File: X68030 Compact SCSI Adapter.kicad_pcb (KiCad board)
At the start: 2 copper layers, 28.8 x 85.3 mm, 5 parts, among them J1 X68030 Internal SCSI Connector, J2 DB25_Plug_MountingHoles

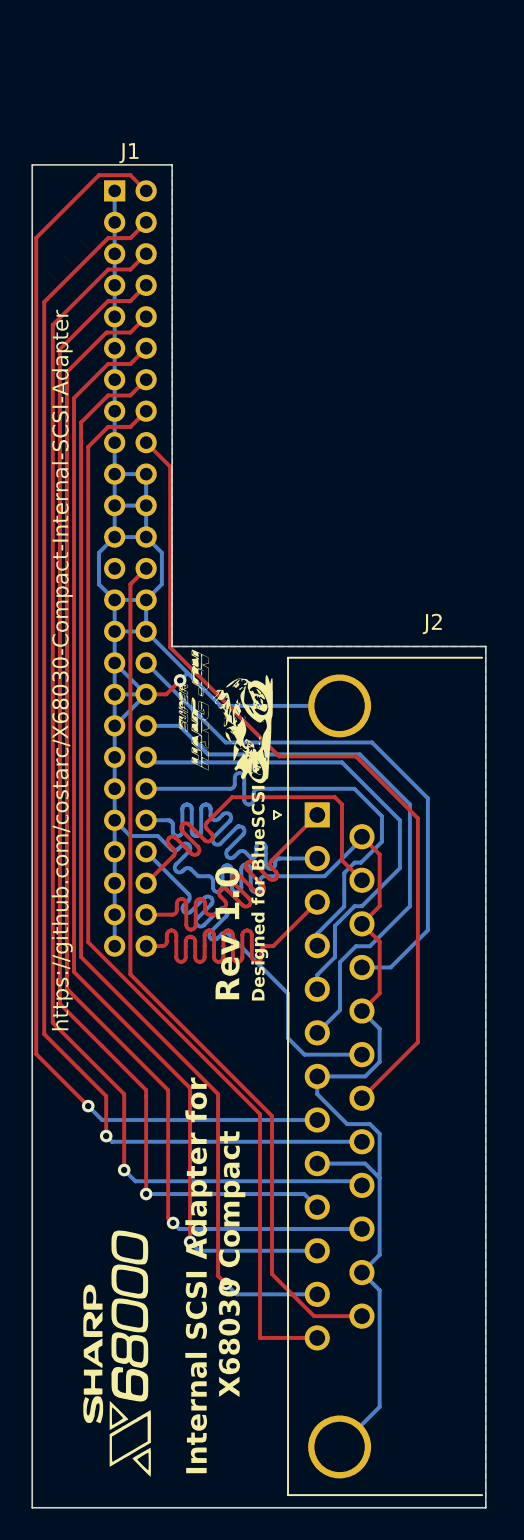
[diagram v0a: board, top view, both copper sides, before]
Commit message: Rev 1.0 - verified to fit
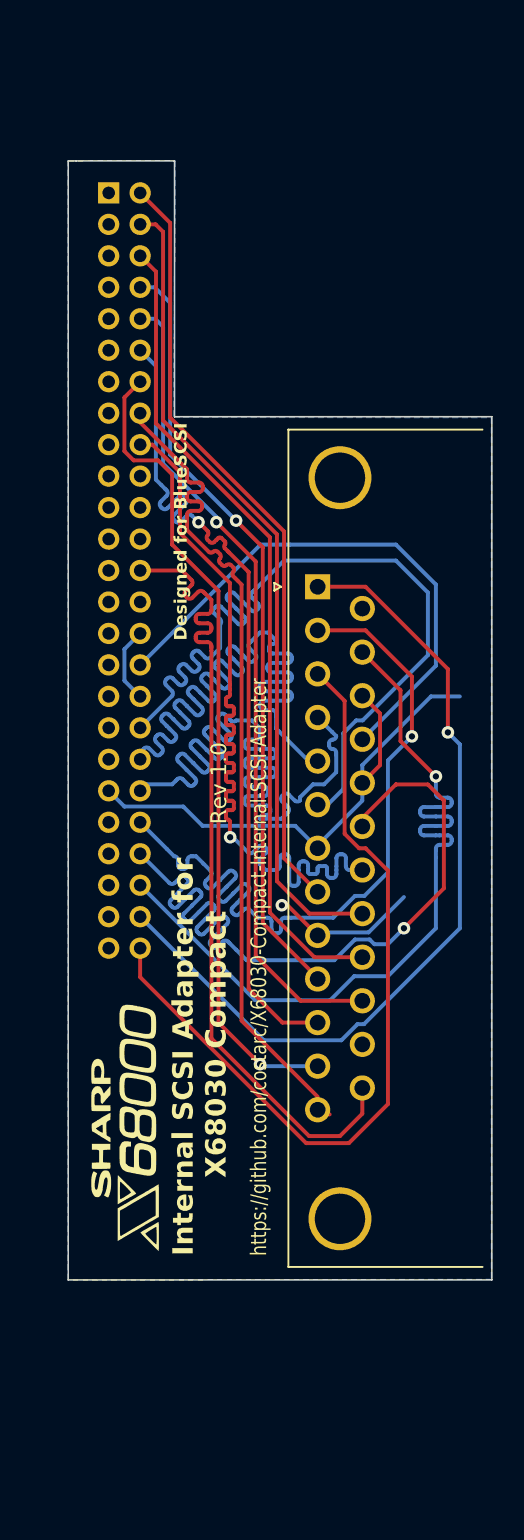
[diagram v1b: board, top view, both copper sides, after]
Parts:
- removed the G*** at (44.5, 63.8)
- removed the G*** at (39.7, 98.8)
- added G***: LOGO, LOGO, B.Cu at (40.9, 92.2)
- moved J2 14.5 mm to (50.4, 56.0)
- moved G*** 14.4 mm to (38.1, 90.4)
- moved J1 0.40 mm to (37.1, 31.0)
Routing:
- net GND: track 176.3 -> 50.3 mm
- net DB0: track 80.5 -> 49.1 mm, vias 1 -> 0
- net DB1: track 79.7 -> 52.2 mm, vias 1 -> 0
- net DB2: track 78.9 -> 52.2 mm, vias 1 -> 0
- net REQ: track 28.3 -> 53.8 mm, vias 0 -> 1
- net DB3: track 74.5 -> 49.2 mm
- net RST: track 29.0 -> 53.8 mm
- net CD: track 27.2 -> 51.9 mm, vias 0 -> 1
- net IO: track 28.1 -> 52.4 mm
- net DB4: track 75.5 -> 52.1 mm
- net MSG: track 27.7 -> 50.5 mm, vias 0 -> 1
- net SEL: track 28.7 -> 50.4 mm, vias 0 -> 1
- net ACK: track 31.0 -> 52.0 mm
- net DB6: track 69.9 -> 52.0 mm
- net DB5: track 71.0 -> 53.9 mm
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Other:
- board size 28.8 x 85.3 mm -> 26.9 x 71.1 mm

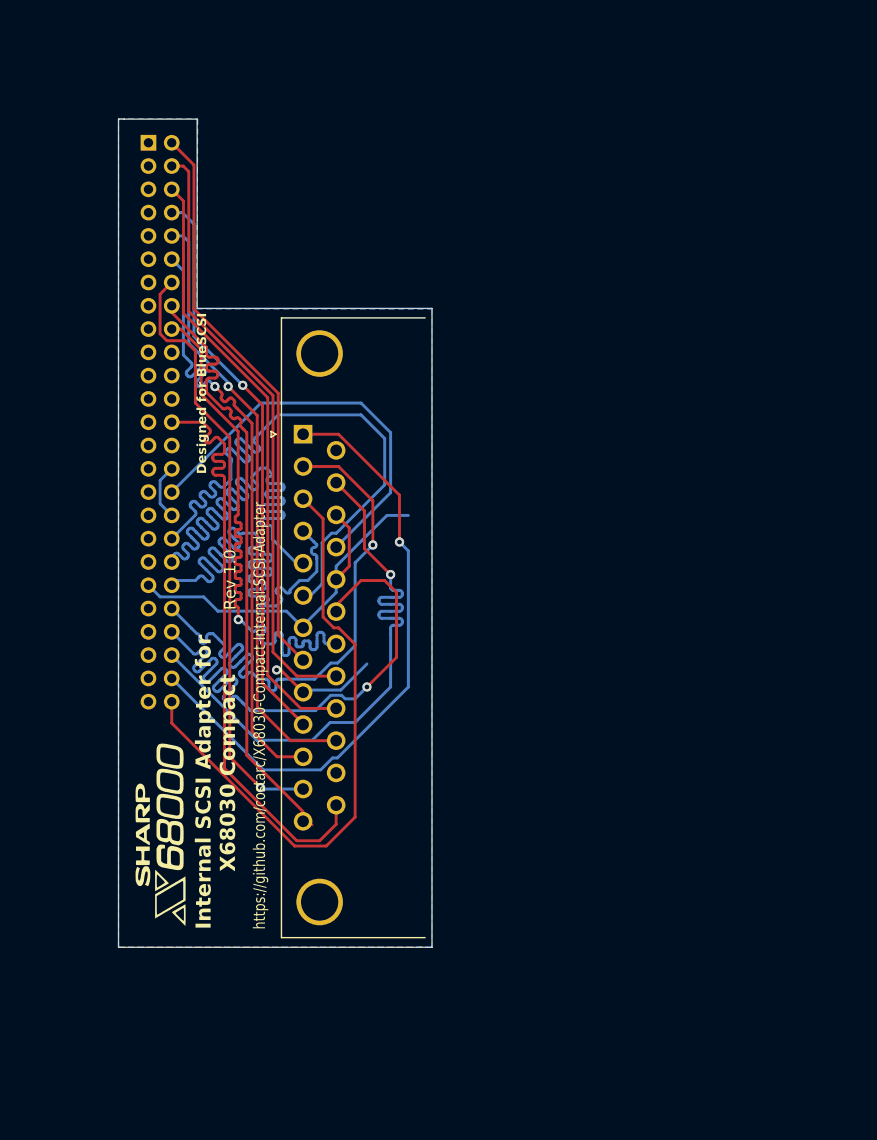
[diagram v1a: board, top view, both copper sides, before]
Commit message: Fabricated
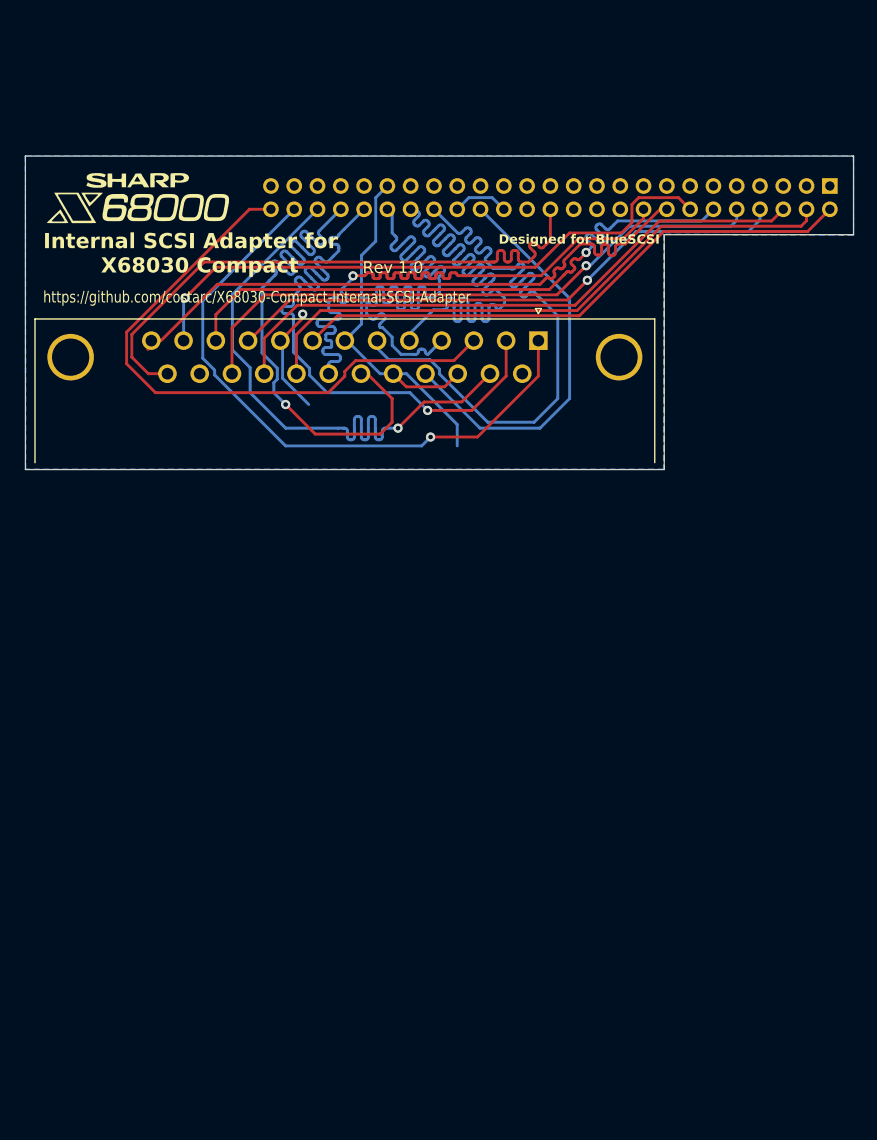
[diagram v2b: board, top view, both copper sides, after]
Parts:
- moved J1 58.6 mm to (95.6, 34.7), turned to 90 degrees
- moved G*** 54.8 mm to (36.2, 35.7), turned to 0 degrees
- moved G*** 54.1 mm to (34.4, 38.4), turned to 180 degrees
- moved J2 21.7 mm to (70.6, 48.0), turned to 0 degrees
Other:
- board size 26.9 x 71.1 mm -> 71.1 x 26.9 mm

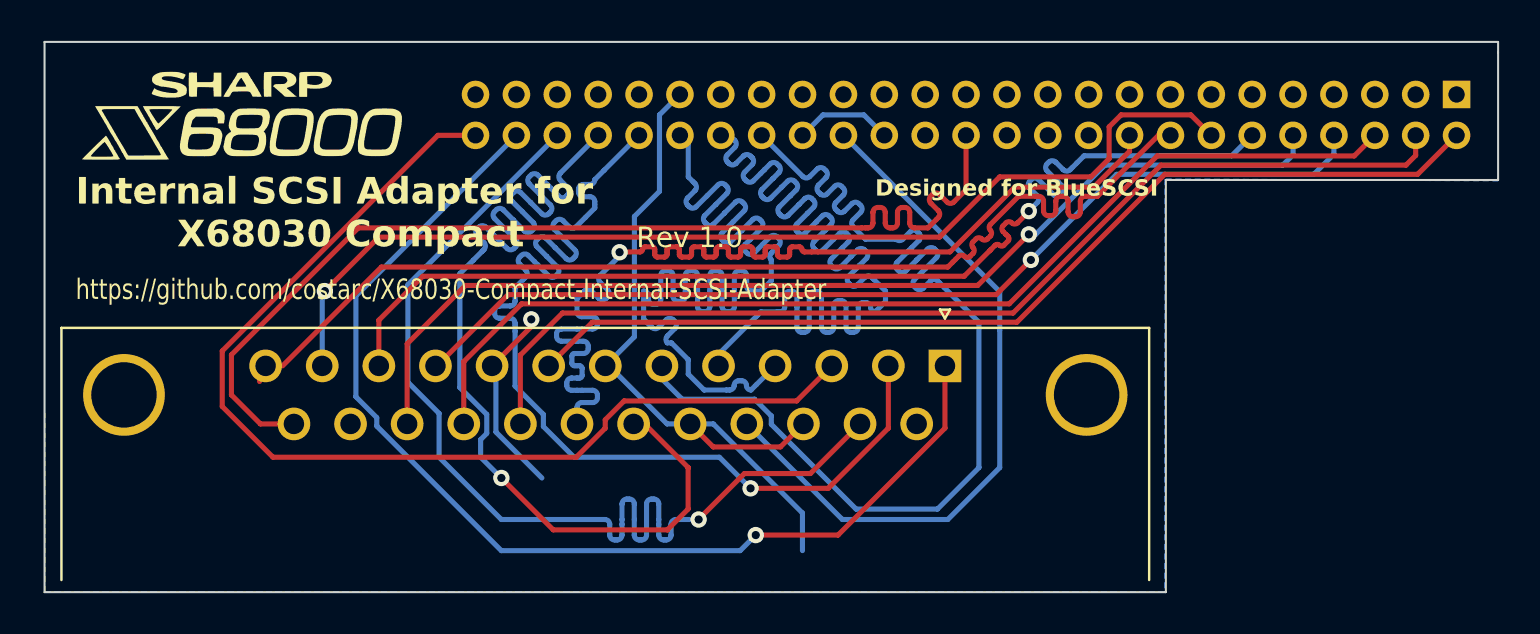
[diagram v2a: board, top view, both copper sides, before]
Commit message: Rev 2.0
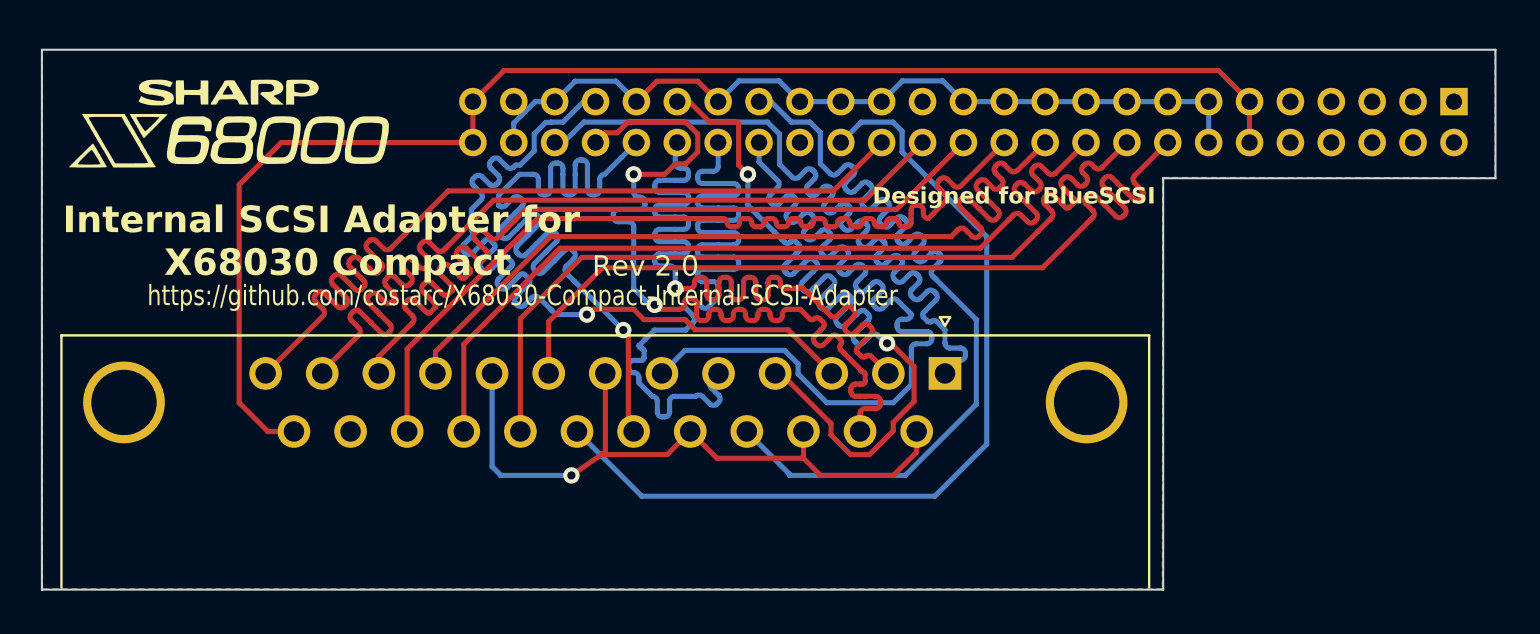
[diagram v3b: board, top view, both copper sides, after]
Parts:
- moved G*** 0.78 mm to (35.1, 38.9)
- moved G*** 0.74 mm to (35.6, 36.1)
- moved J1 0.37 mm to (95.5, 35.1)
- moved J2 0.37 mm to (70.6, 48.3)
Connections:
- J1 pad 1: GND -> unconnected-(J1-Pin_1-Pad1)
- J1 pad 10: DB4 -> unconnected-(J1-Pin_10-Pad10)
- J1 pad 11: GND -> VCC
- J1 pad 12: DB5 -> VCC
- J1 pad 14: DB6 -> GND
- J1 pad 16: DB7 -> DB0
- J1 pad 18: DBP -> DB1
- J1 pad 2: DB0 -> unconnected-(J1-Pin_2-Pad2)
- J1 pad 20: GND -> DB2
- J1 pad 22: GND -> DB3
- J1 pad 24: GND -> DB4
- J1 pad 25: unconnected-(J1-Pin_25-Pad25) -> GND
- J1 pad 26: +5V -> DB5
- J1 pad 27: GND -> unconnected-(J1-Pin_27-Pad27)
- J1 pad 28: GND -> DB6
- J1 pad 3: GND -> unconnected-(J1-Pin_3-Pad3)
- J1 pad 30: GND -> DB7
- J1 pad 32: ATN -> DBP
- J1 pad 34: GND -> TMPWR
- J1 pad 35: GND -> ATN
- J1 pad 39: GND -> RST
- J1 pad 4: DB1 -> unconnected-(J1-Pin_4-Pad4)
- J1 pad 40: RST -> MSG
- J1 pad 42: MSG -> SEL
- J1 pad 43: GND -> IO
- J1 pad 44: SEL -> CD
- J1 pad 46: CD -> REQ
- J1 pad 48: REQ -> GND
- J1 pad 49: GND -> VCC
- J1 pad 5: GND -> ID1
- J1 pad 50: IO -> VCC
- J1 pad 6: DB2 -> ID2
- J1 pad 7: GND -> ID4
- J1 pad 8: DB3 -> HD LED
- J1 pad 9: GND -> unconnected-(J1-Pin_9-Pad9)
- J2 pad 25: +5V -> VCC
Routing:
- net VCC: track 0.00 -> 69.5 mm
- net +5V: track 52.2 -> 0.00 mm
- net GND: track 50.3 -> 75.6 mm
- net REQ: track 53.8 -> 40.4 mm, vias 1 -> 0
- net ACK: track 52.0 -> 40.3 mm
- net IO: track 52.4 -> 41.9 mm, vias 0 -> 1
- net RST: track 53.8 -> 43.2 mm, vias 0 -> 2
- net DB5: track 53.9 -> 43.4 mm, vias 1 -> 0
- net MSG: track 50.5 -> 40.1 mm
- net BSY: track 52.9 -> 42.9 mm
- net DB7: track 53.5 -> 43.5 mm
- net CD: track 51.9 -> 42.1 mm, vias 1 -> 2
- net DB1: track 52.2 -> 43.2 mm
- net DB2: track 52.2 -> 43.4 mm
- net DB4: track 52.1 -> 43.3 mm, vias 1 -> 0
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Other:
- board size 71.1 x 26.9 mm -> 71.1 x 26.4 mm
- board text added: "Rev 2.0"
- board text removed: "Rev 1.0"
